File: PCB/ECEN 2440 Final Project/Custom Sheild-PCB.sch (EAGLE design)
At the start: 7 parts

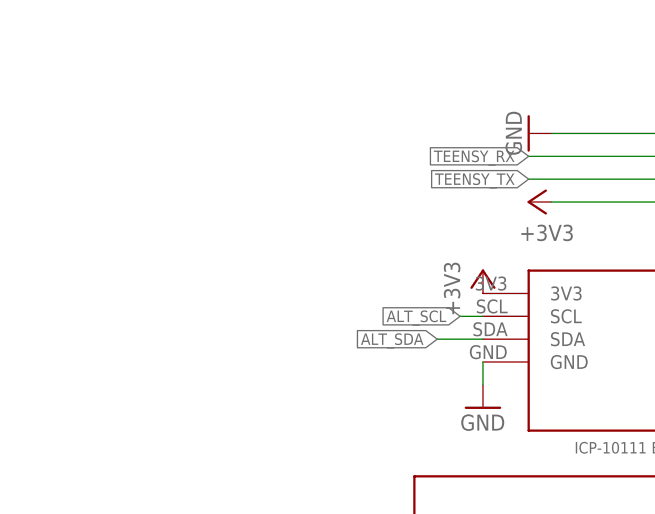
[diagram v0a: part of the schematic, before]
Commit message: New changes to pcb board
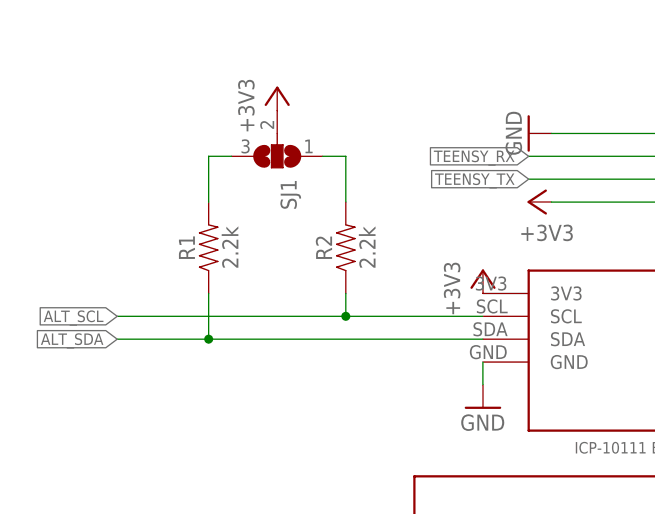
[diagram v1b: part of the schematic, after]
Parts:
- added R1, R2: 2.2k, SparkFun-Resistors:2.2KOHM-0603-1/10W-1%
- added SJ1: (no value), jumper:SJ2W
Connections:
- new net N$1: R1.2, SJ1.3
- new net N$2: R2.2, SJ1.1
- net +3V3: now also SJ1.2
- net ALT_SCL: now also R2.1
- net ALT_SDA: now also R1.1
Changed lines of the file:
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@@
 <part name="+3V4" library="supply1" library_urn="urn:adsk.eagle:library:371" deviceset="+3V3" device=""/>
 <part name="GND3" library="supply1" library_urn="urn:adsk.eagle:library:371" deviceset="GND" device=""/>
+<part name="SJ1" library="jumper" library_urn="urn:adsk.eagle:library:252" deviceset="SJ2W" device="" package3d_urn="urn:adsk.eagle:package:15474/1"/>
+<part name="R1" library="SparkFun-Resistors" library_urn="urn:adsk.eagle:library:532" deviceset="2.2KOHM" device="-0603-1/10W-1%" package3d_urn="urn:adsk.eagle:package:39650/1" value="2.2k"/>
+<part name="R2" library="SparkFun-Resistors" library_urn="urn:adsk.eagle:library:532" deviceset="2.2KOHM" device="-0603-1/10W-1%" package3d_urn="urn:adsk.eagle:package:39650/1" value="2.2k"/>
+<part name="+3V6" library="supply1" library_urn="urn:adsk.eagle:library:371" deviceset="+3V3" device=""/>
 </parts>
 <sheets>
@@
 <attribute name="VALUE" x="0" y="-40.64" size="1.778" layer="96" rot="R90"/>
 </instance>
+<instance part="SJ1" gate="G$1" x="-22.86" y="101.6" smashed="yes" rot="R270">
+<attribute name="NAME" x="-22.479" y="99.06" size="1.778" layer="95" rot="R270"/>
+<attribute name="VALUE" x="-24.765" y="99.06" size="1.778" layer="96" rot="R270"/>
+</instance>
+<instance part="R1" gate="G$1" x="-30.48" y="91.44" smashed="yes" rot="R90">
+<attribute name="NAME" x="-32.004" y="91.44" size="1.778" layer="95" font="vector" rot="R90" align="bottom-center"/>
+<attribute name="VALUE" x="-28.956" y="91.44" size="1.778" layer="96" font="vector" rot="R90" align="top-center"/>
+</instance>
+<instance part="R2" gate="G$1" x="-15.24" y="91.44" smashed="yes" rot="R90">
+<attribute name="NAME" x="-16.764" y="91.44" size="1.778" layer="95" font="vector" rot="R90" align="bottom-center"/>
+<attribute name="VALUE" x="-13.716" y="91.44" size="1.778" layer="96" font="vector" rot="R90" align="top-center"/>
+</instance>
+<instance part="+3V6" gate="G$1" x="-22.86" y="109.22" smashed="yes">
+<attribute name="VALUE" x="-25.4" y="104.14" size="1.778" layer="96" rot="R90"/>
+</instance>
 </instances>
 <busses>
@@
 <segment>
 <pinref part="U$2" gate="G$1" pin="SDA"/>
-<wire x1="-5.08" y1="81.28" x2="0" y2="81.28" width="0.1524" layer="91"/>
-<label x="-5.08" y="81.28" size="1.27" layer="95" rot="R180" xref="yes"/>
+<wire x1="-40.64" y1="81.28" x2="-30.48" y2="81.28" width="0.1524" layer="91"/>
+<label x="-40.64" y="81.28" size="1.27" layer="95" rot="R180" xref="yes"/>
+<pinref part="R1" gate="G$1" pin="1"/>
+<wire x1="-30.48" y1="81.28" x2="0" y2="81.28" width="0.1524" layer="91"/>
+<wire x1="-30.48" y1="81.28" x2="-30.48" y2="86.36" width="0.1524" layer="91"/>
+<junction x="-30.48" y="81.28"/>
 </segment>
 <segment>
@@
 <segment>
 <pinref part="U$2" gate="G$1" pin="SCL"/>
-<wire x1="-2.54" y1="83.82" x2="0" y2="83.82" width="0.1524" layer="91"/>
-<label x="-2.54" y="83.82" size="1.27" layer="95" rot="R180" xref="yes"/>
+<wire x1="-40.64" y1="83.82" x2="-15.24" y2="83.82" width="0.1524" layer="91"/>
+<label x="-40.64" y="83.82" size="1.27" layer="95" rot="R180" xref="yes"/>
+<pinref part="R2" gate="G$1" pin="1"/>
+<wire x1="-15.24" y1="83.82" x2="0" y2="83.82" width="0.1524" layer="91"/>
+<wire x1="-15.24" y1="86.36" x2="-15.24" y2="83.82" width="0.1524" layer="91"/>
+<junction x="-15.24" y="83.82"/>
 </segment>
 <segment>
@@
 <pinref part="+3V4" gate="G$1" pin="+3V3"/>
 </segment>
+<segment>
+<pinref part="SJ1" gate="G$1" pin="2"/>
+<pinref part="+3V6" gate="G$1" pin="+3V3"/>
+</segment>
 </net>
 <net name="CD1" class="0">
@@
 </segment>
 </net>
+<net name="N$1" class="0">
+<segment>
+<pinref part="R1" gate="G$1" pin="2"/>
+<wire x1="-30.48" y1="96.52" x2="-30.48" y2="101.6" width="0.1524" layer="91"/>
+<pinref part="SJ1" gate="G$1" pin="3"/>
+<wire x1="-30.48" y1="101.6" x2="-27.94" y2="101.6" width="0.1524" layer="91"/>
+</segment>
+</net>
+<net name="N$2" class="0">
+<segment>
+<pinref part="SJ1" gate="G$1" pin="1"/>
+<wire x1="-17.78" y1="101.6" x2="-15.24" y2="101.6" width="0.1524" layer="91"/>
+<pinref part="R2" gate="G$1" pin="2"/>
+<wire x1="-15.24" y1="101.6" x2="-15.24" y2="96.52" width="0.1524" layer="91"/>
+</segment>
+</net>
